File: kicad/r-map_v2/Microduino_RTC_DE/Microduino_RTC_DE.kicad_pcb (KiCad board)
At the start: 2 copper layers, 25.5 x 27.9 mm, 16 parts, among them P1 CONN_1x27, U1 PCF8563, Y1 32,762 kHz

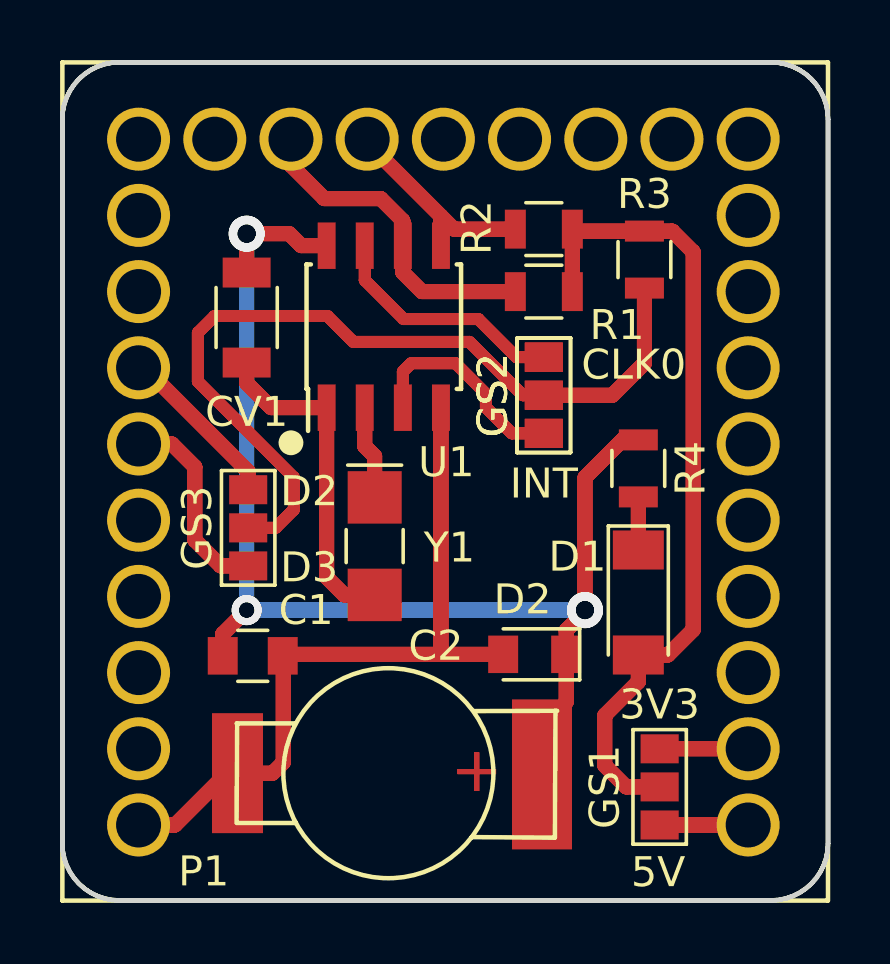
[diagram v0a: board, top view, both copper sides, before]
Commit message: update kicad project
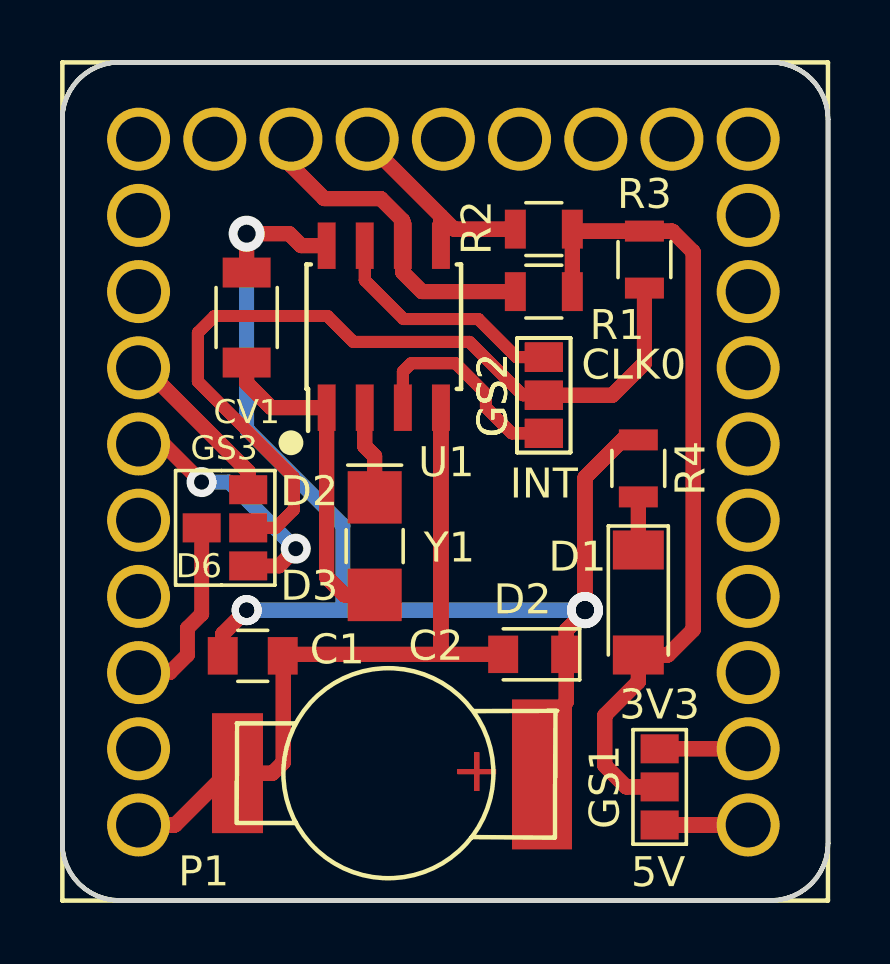
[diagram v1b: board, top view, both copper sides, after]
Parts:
- GS3: value GS3 -> GS4; footprint Connectors:GS3 -> Libreria_PCB_mia:GS4
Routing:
- net Net-(C1-Pad1): track 87.2 -> 76.0 mm, vias 6 -> 5
- net /D6: track 0.00 -> 6.31 mm
- net /D3: track 13.5 -> 8.52 mm, vias 0 -> 2
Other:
- board text added: "D6"
